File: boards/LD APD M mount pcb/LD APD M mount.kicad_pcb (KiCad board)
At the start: 2 copper layers, 101.2 x 15 mm, 13 parts, among them J3 Conn_01x10, U1 SensL_SiPM

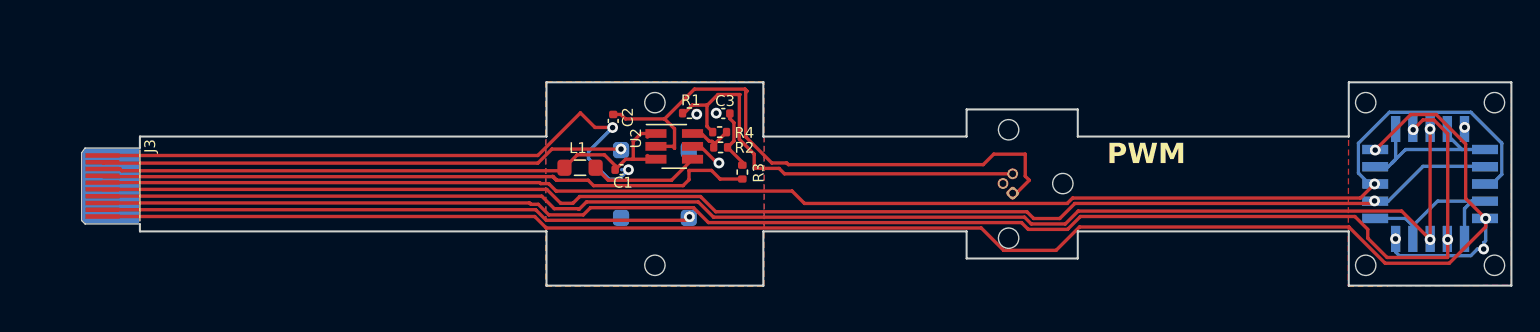
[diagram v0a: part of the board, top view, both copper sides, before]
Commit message: made macro system pcb v2
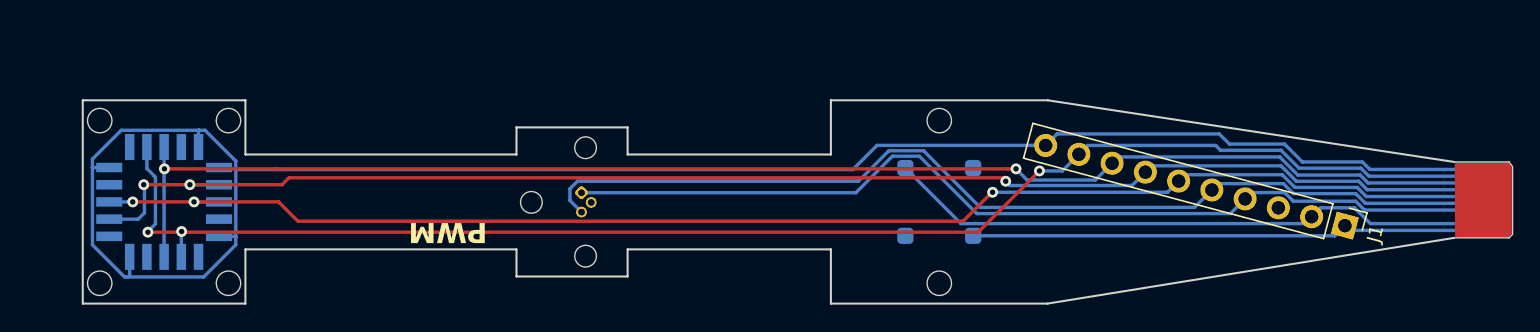
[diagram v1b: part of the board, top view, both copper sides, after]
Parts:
- removed C1, C2: 1u, Capacitor_SMD:C_0402_1005Metric
- removed C3: 0.1u, Capacitor_SMD:C_0402_1005Metric
- removed L1: 4.7u, Inductor_SMD:L_0805_2012Metric_Pad1.05x1.20mm_HandSolder
- removed R1: 2, Resistor_SMD:R_0402_1005Metric
- removed R2, R4: 4.7k, Resistor_SMD:R_0402_1005Metric
- removed R3: 33k, Resistor_SMD:R_0402_1005Metric
- removed U2: ~, Package_TO_SOT_SMD:SOT-23-6_Handsoldering
- added J1: Conn_01x10, Connector_PinHeader_2.54mm:PinHeader_1x10_P2.54mm_Vertical, F.Cu at (187.2, 91.3)
- J3: moved to B.Cu
- moved J3 100.5 mm to (197.0, 89.5)
- moved U3 93.4 mm to (100.0, 89.6), turned to -90 degrees
- moved LD1 31.2 mm to (131.1, 88.9), turned to -90 degrees
- moved U1 21.0 mm to (157.2, 89.6)
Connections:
- J3 pad 1: Net-(J3-Pin_1) -> /SiPM-
- J3 pad 2: Net-(J3-Pin_2) -> Net-(J1-Pin_2)
- J3 pad 3: Net-(J3-Pin_3) -> unconnected-(J3-Pin_3-Pad3)
- J3 pad 4: Net-(J3-Pin_4) -> Net-(J1-Pin_4)
- J3 pad 5: Net-(J3-Pin_5) -> Net-(J1-Pin_5)
- J3 pad 7: Net-(J3-Pin_7) -> Net-(J1-Pin_7)
- J3 pad 8: Net-(J3-Pin_8) -> Net-(J1-Pin_8)
- J3 pad 9: Net-(J3-Pin_9) -> /X-
- LD1 pad 1: Net-(LD1-A) -> Net-(J1-Pin_4)
- LD1 pad 3: Net-(LD1-C) -> Net-(J1-Pin_5)
- U1 pad 1: Net-(J3-Pin_2) -> /SiPM-
- U1 pad 3: Net-(J3-Pin_9) -> Net-(J1-Pin_2)
- U1 pad 4: (no net) -> unconnected-(U1-NC-Pad4)
- U3 pad 10: Net-(J3-Pin_5) -> Net-(J1-Pin_7)
- U3 pad 12: Net-(U3-NC-Pad12) -> unconnected-(U3-NC-Pad12)
- U3 pad 13: Net-(J3-Pin_1) -> GND
- U3 pad 14: Net-(U3-NC-Pad12) -> unconnected-(U3-NC-Pad14)
- U3 pad 15: Net-(J3-Pin_3) -> /X-
- U3 pad 16: Net-(J3-Pin_4) -> Net-(J1-Pin_8)
- U3 pad 17: Net-(U3-NC-Pad12) -> unconnected-(U3-NC-Pad17)
- U3 pad 18: Net-(J3-Pin_1) -> GND
- U3 pad 19: Net-(U3-NC-Pad12) -> unconnected-(U3-NC-Pad19)
- U3 pad 2: Net-(U3-NC-Pad12) -> unconnected-(U3-NC-Pad2)
- U3 pad 20: Net-(J3-Pin_5) -> Net-(J1-Pin_7)
- U3 pad 3: Net-(J3-Pin_1) -> GND
- U3 pad 4: Net-(U3-NC-Pad12) -> unconnected-(U3-NC-Pad4)
- U3 pad 5: Net-(J3-Pin_3) -> /X-
- U3 pad 6: Net-(J3-Pin_4) -> Net-(J1-Pin_8)
- U3 pad 7: Net-(U3-NC-Pad12) -> unconnected-(U3-NC-Pad7)
- U3 pad 8: Net-(J3-Pin_1) -> GND
- U3 pad 9: Net-(U3-NC-Pad12) -> unconnected-(U3-NC-Pad9)
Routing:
- net Net-(J3-Pin_1): track 131.5 -> 0.00 mm, vias 5 -> 0
- net Net-(J3-Pin_3): track 114.9 -> 0.00 mm, vias 2 -> 0
- net /X-: track 0.00 -> 111.6 mm, vias 0 -> 3
- net Net-(J3-Pin_4): track 108.7 -> 0.00 mm, vias 2 -> 0
- net Net-(J1-Pin_7): track 0.00 -> 108.5 mm, vias 0 -> 3
- net Net-(J1-Pin_8): track 0.00 -> 107.9 mm, vias 0 -> 2
- net Net-(J3-Pin_5): track 104.9 -> 0.00 mm, vias 1 -> 0
- net GND: track 49.3 -> 137.0 mm, vias 5 -> 0
- net Net-(J1-Pin_5): track 0.00 -> 74.3 mm
- net Net-(J1-Pin_4): track 0.00 -> 71.2 mm
- net Net-(J3-Pin_7): track 49.1 -> 0.00 mm
- net Net-(J3-Pin_8): track 47.1 -> 0.00 mm
- net Net-(J1-Pin_2): track 0.00 -> 45.9 mm
- net Net-(LD1-A): track 44.1 -> 0.00 mm
- net Net-(J3-Pin_2): track 43.7 -> 0.00 mm, vias 1 -> 0
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- removed copper zone on B.Cu, net GND
- removed copper zone on F.Cu, net GND
- removed copper zone on F.Cu, net Net-(J3-Pin_1)
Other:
- outline, holes or cut-outs redrawn
